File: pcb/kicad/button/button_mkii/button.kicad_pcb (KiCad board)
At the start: 2 copper layers, 163 parts, among them J1 SWD with less, U1 STBlueNRG-1, U2 TLV1117LV-3V, Y1 Xtal 32.768kHz, Y2 XTAL 32MHz

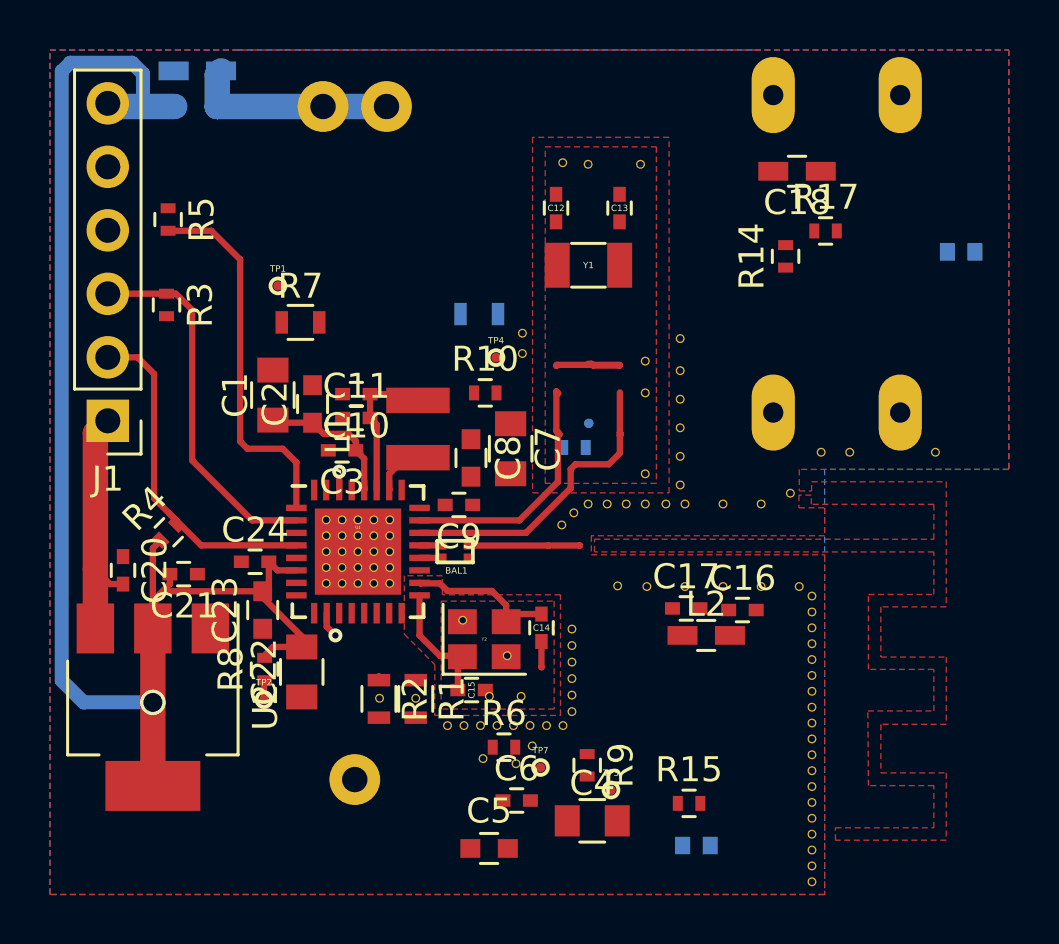
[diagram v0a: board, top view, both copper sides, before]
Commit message: rev3 prog, almost there...
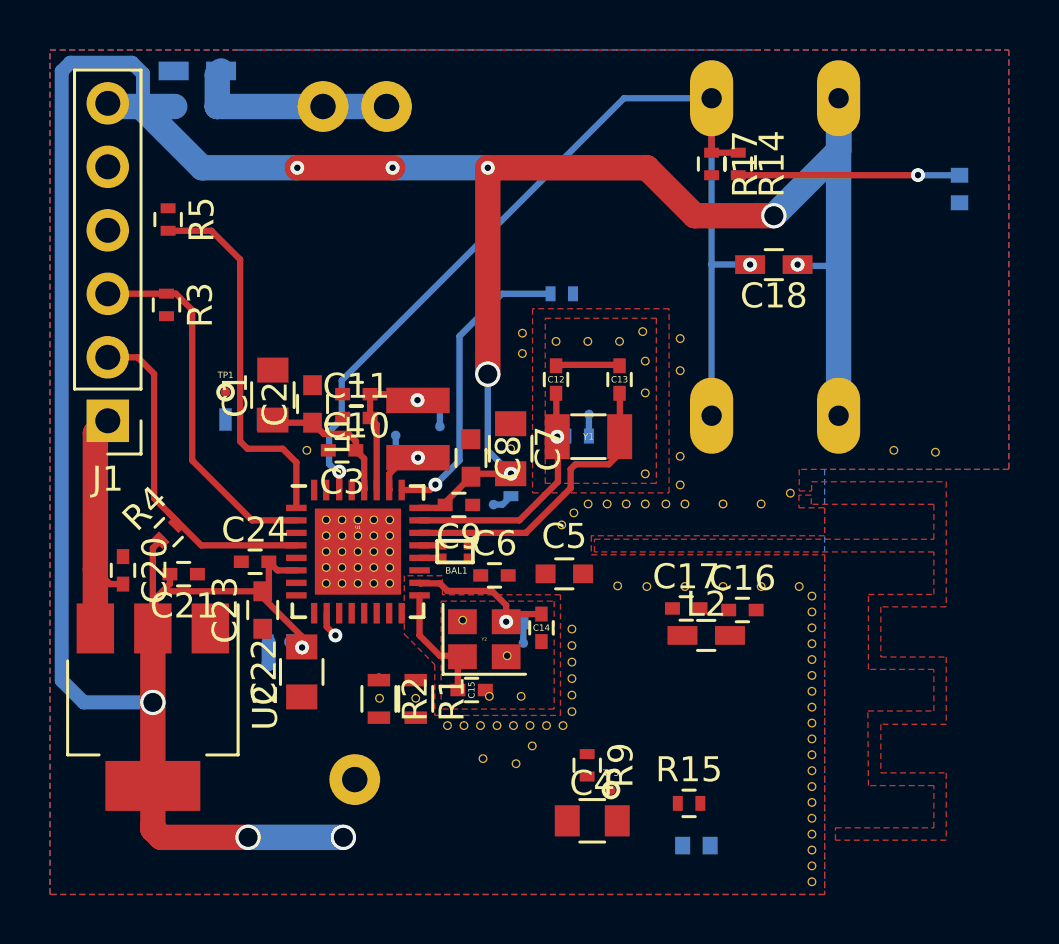
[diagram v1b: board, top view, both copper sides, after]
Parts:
- R10, R6, R7, R8, TP2, TP4, TP7: moved to B.Cu
- R13: footprint Resistors_SMD:R_0603 -> Resistors_SMD:R_0402
- moved REF** 21.7 mm to (119.6, 100.2)
- moved REF** 12.4 mm to (127.8, 100.2)
- moved C5 11.4 mm to (129.9, 105.2)
- moved C6 9.05 mm to (127.1, 105.2)
- moved REF** 8.59 mm to (143.1, 100.2)
- moved REF** 7.16 mm to (129.6, 95.9)
- moved REF** 7.14 mm to (132.1, 95.9)
- moved REF** 7.09 mm to (130.9, 95.9)
- moved C12 6.86 mm to (129.6, 97.4)
- moved C13 6.86 mm to (132.1, 97.4)
- moved Y1 6.86 mm to (130.9, 99.7)
- moved TP4 5.88 mm to (127.1, 102.4), turned to 90 degrees
- moved R17 5.29 mm to (135.8, 88.8), turned to 270 degrees
- moved R6 5.03 mm to (127.8, 107.1)
- moved TP7 5.03 mm to (128.3, 107.9)
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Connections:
- U2 pad 4: (no net) -> +3V3
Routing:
- net +3V3: track 60.2 -> 145.4 mm, vias 1 -> 11
- net /DIO12_BUTTON: track 0.74 -> 41.8 mm, vias 1 -> 2
- net Net-(R13-Pad2): track 0.00 -> 12.1 mm, vias 0 -> 1
- net Net-(D1-Pad2): track 0.00 -> 8.86 mm, vias 0 -> 1
- net (no net): track 5.02 -> 0.00 mm
- net Net-(BAL1-Pad3): track 3.29 -> 0.00 mm
- net GND: track 17.3 -> 18.8 mm
- net Net-(R12-Pad1): track 0.00 -> 1.06 mm
- net Net-(R11-Pad2): track 0.00 -> 0.90 mm
- net Net-(R16-Pad2): track 0.00 -> 0.87 mm
- net Net-(R6-Pad2): track 0.00 -> 0.85 mm
- net Net-(R10-Pad2): track 0.00 -> 0.84 mm
- net Net-(C12-Pad2): track 10.1 -> 10.9 mm, vias 0 -> 1
- net Net-(C14-Pad2): track 6.14 -> 6.35 mm, vias 0 -> 1
- net Net-(L1-Pad1): track 2.09 -> 2.11 mm, vias 0 -> 1
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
